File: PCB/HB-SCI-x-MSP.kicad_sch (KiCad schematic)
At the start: 31 parts, among them J1 Prog, J2 FTDI, Q1 BC858, SW1 Config, SW2 4x SW, U1 ATmega328P-AU, U2 MSP430F2001IPW, U3 CC1101, Y1 32kHz

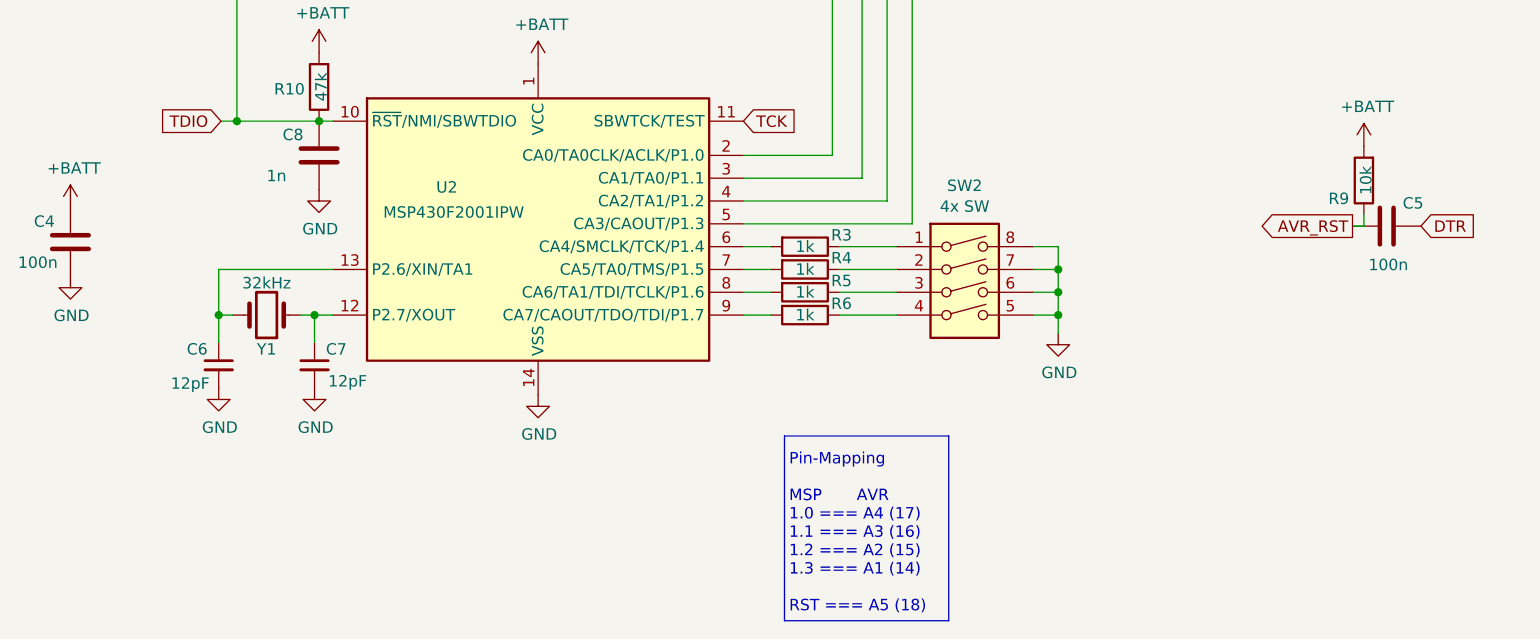
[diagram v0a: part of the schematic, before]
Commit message: update kicad
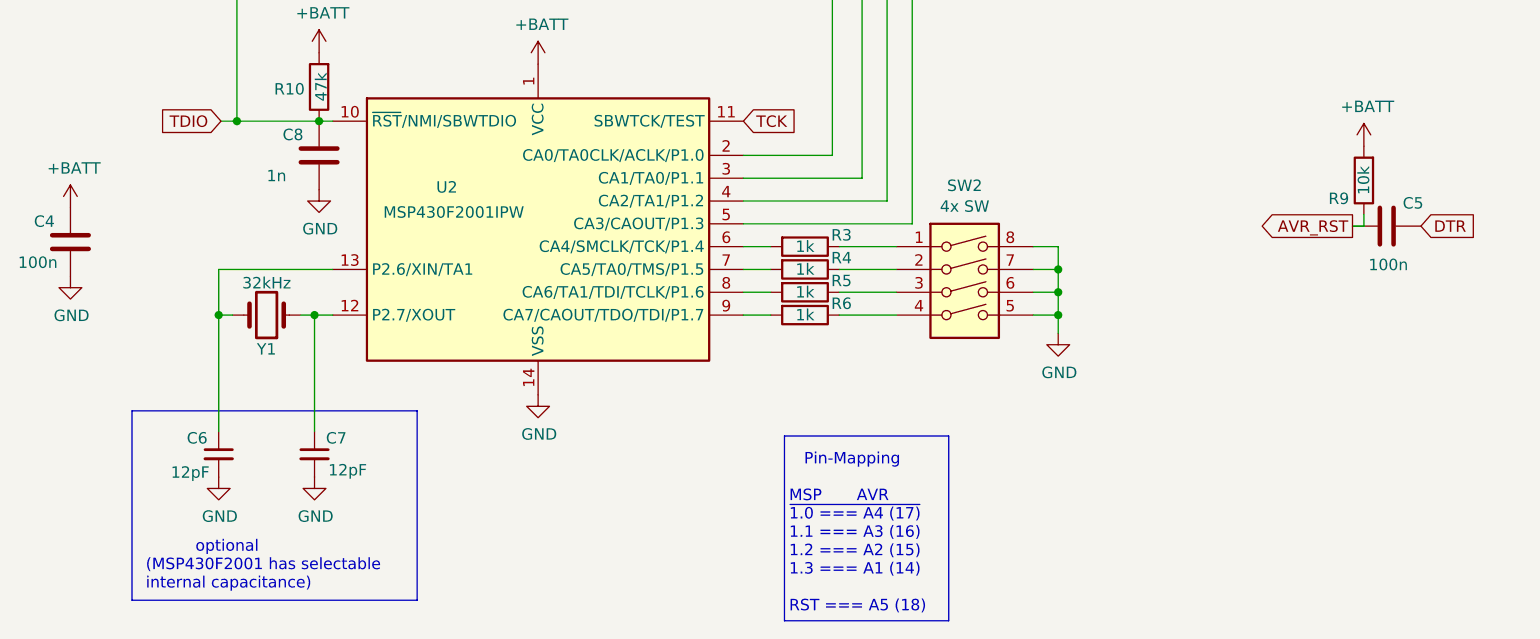
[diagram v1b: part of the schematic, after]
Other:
- note added: "Pin-Mapping MSP AVR ~{1.0 === A4 (17)} 1.1 === A3 (16) 1.2 === A2 (15) 1.3 === A1 (14) RST === A5 (18)"
- note added: "optional (MSP430F2001 has selectable internal capacitance)"
- note removed: "Pin-Mapping MSP AVR 1.0 === A4 (17) 1.1 === A3 (16) 1.2 === A2 (15) 1.3 === A1 (14) RST === A5 (18)"
- moved on the sheet: C6, C7
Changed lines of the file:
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@@
 (kicad_sch (version 20210621) (generator eeschema)
   (paper "A4")
-  (junction (at 43.688 137.668) (diameter 0) (color 0 0 0 0))
-  (junction (at 184.404 110.49) (diameter 0) (color 0 0 0 0))
-  (junction (at 177.546 48.006) (diameter 0) (color 0 0 0 0))
-  (junction (at 213.614 60.706) (diameter 0) (color 0 0 0 0))
-  (junction (at 52.324 159.258) (diameter 0) (color 0 0 0 0))
-  (junction (at 76.962 37.846) (diameter 0) (color 0 0 0 0))
-  (junction (at 79.502 37.846) (diameter 0) (color 0 0 0 0))
-  (junction (at 135.128 154.178) (diameter 0) (color 0 0 0 0))
   (junction (at 135.128 156.718) (diameter 0) (color 0 0 0 0))
   (junction (at 124.714 69.088) (diameter 0) (color 0 0 0 0))
   (junction (at 135.128 159.258) (diameter 0) (color 0 0 0 0))
-  (junction (at 52.832 137.668) (diameter 0) (color 0 0 0 0))
-  (junction (at 41.656 159.258) (diameter 0) (color 0 0 0 0))
+  (junction (at 184.404 110.49) (diameter 0) (color 0 0 0 0))
+  (junction (at 43.688 137.668) (diameter 0) (color 0 0 0 0))
+  (junction (at 52.324 159.258) (diameter 0) (color 0 0 0 0))
+  (junction (at 177.546 48.006) (diameter 0) (color 0 0 0 0))
+  (junction (at 79.502 37.846) (diameter 0) (color 0 0 0 0))
   (junction (at 177.546 61.976) (diameter 0) (color 0 0 0 0))
   (junction (at 177.546 41.148) (diameter 0) (color 0 0 0 0))
+  (junction (at 41.656 159.258) (diameter 0) (color 0 0 0 0))
+  (junction (at 76.962 37.846) (diameter 0) (color 0 0 0 0))
+  (junction (at 52.832 137.668) (diameter 0) (color 0 0 0 0))
+  (junction (at 213.614 60.706) (diameter 0) (color 0 0 0 0))
+  (junction (at 135.128 154.178) (diameter 0) (color 0 0 0 0))
   (no_connect (at 92.202 107.188))
   (no_connect (at 206.502 55.626))
@@
     (stroke (width 0) (type default) (color 0 0 0 0))
   )
-  (wire (pts (xy 41.656 159.258) (xy 41.656 162.306))
+  (wire (pts (xy 41.656 159.258) (xy 41.656 172.212))
     (stroke (width 0) (type default) (color 0 0 0 0))
   )
@@
     (stroke (width 0) (type default) (color 0 0 0 0))
   )
+  (polyline (pts (xy 32.004 169.926) (xy 32.004 191.008))
+    (stroke (width 0) (type default) (color 0 0 0 0))
+  )
+  (polyline (pts (xy 32.004 169.926) (xy 63.754 169.926))
+    (stroke (width 0) (type default) (color 0 0 0 0))
+  )
+  (polyline (pts (xy 63.754 191.008) (xy 32.004 191.008))
+    (stroke (width 0) (type default) (color 0 0 0 0))
+  )
+  (polyline (pts (xy 63.754 169.926) (xy 63.754 191.008))
+    (stroke (width 0) (type default) (color 0 0 0 0))
+  )
   (wire (pts (xy 132.334 151.638) (xy 135.128 151.638))
     (stroke (width 0) (type default) (color 0 0 0 0))
@@
     (stroke (width 0) (type default) (color 0 0 0 0))
   )
-  (wire (pts (xy 52.324 162.306) (xy 52.324 159.258))
+  (wire (pts (xy 52.324 172.212) (xy 52.324 159.258))
     (stroke (width 0) (type default) (color 0 0 0 0))
   )
@@
     (stroke (width 0) (type default) (color 0 0 0 0))
   )
-  (text "Pin-Mapping\n\nMSP       AVR\n1.0 === A4 (17)\n1.1 === A3 (16)\n1.2 === A2 (15)\n1.3 === A1 (14)\n\nRST === A5 (18)"
+  (text "   Pin-Mapping\n\nMSP       AVR\n~{1.0 === A4 (17)}\n1.1 === A3 (16)\n1.2 === A2 (15)\n1.3 === A1 (14)\n\nRST === A5 (18)"
     (at 105.156 192.532 0)
+    (effects (font (size 1.27 1.27)) (justify left bottom))
+  )
+  (text "          optional\n(MSP430F2001 has selectable \ninternal capacitance)"
+    (at 33.528 189.992 0)
     (effects (font (size 1.27 1.27)) (justify left bottom))
   )
@@
     (in_bom yes) (on_board yes)
     (property "Reference" "R9" (id 0) (at 166.37 146.304 0))
-    (property "Value" "10k" (id 1) (at 169.418 144.272 90))
+    (property "Value" "10k" (id 1) (at 169.164 144.272 90))
     (property "Footprint" "Resistor_SMD:R_0805_2012Metric_Pad1.15x1.40mm_HandSolder" (id 2) (at 170.942 144.272 90)
       (effects (font (size 1.27 1.27)) hide)
@@
     (pin "1")
   )
-  (symbol (lib_id "Device:C_Small") (at 41.656 164.846 0) (unit 1)
-    (in_bom yes) (on_board yes)
-    (property "Reference" "C6" (id 0) (at 38.1 163.068 0)
-      (effects (font (size 1.27 1.27)) (justify left))
-    )
-    (property "Value" "12pF" (id 1) (at 36.322 166.878 0)
-      (effects (font (size 1.27 1.27)) (justify left))
-    )
-    (property "Footprint" "Capacitor_SMD:C_0805_2012Metric_Pad1.15x1.40mm_HandSolder" (id 2) (at 41.656 164.846 0)
-      (effects (font (size 1.27 1.27)) hide)
-    )
-    (property "Datasheet" "~" (id 3) (at 41.656 164.846 0)
-      (effects (font (size 1.27 1.27)) hide)
-    )
-    (pin "1")
-    (pin "2")
-  )
-  (symbol (lib_id "Device:C_Small") (at 52.324 164.846 0) (unit 1)
-    (in_bom yes) (on_board yes)
-    (property "Reference" "C7" (id 0) (at 53.594 163.068 0)
-      (effects (font (size 1.27 1.27)) (justify left))
-    )
-    (property "Value" "12pF" (id 1) (at 53.848 166.624 0)
-      (effects (font (size 1.27 1.27)) (justify left))
-    )
-    (property "Footprint" "Capacitor_SMD:C_0805_2012Metric_Pad1.15x1.40mm_HandSolder" (id 2) (at 52.324 164.846 0)
-      (effects (font (size 1.27 1.27)) hide)
-    )
-    (property "Datasheet" "~" (id 3) (at 52.324 164.846 0)
-      (effects (font (size 1.27 1.27)) hide)
-    )
-    (pin "1")
-    (pin "2")
-  )
-  (symbol (lib_id "power:GND") (at 41.656 167.386 0) (unit 1)
-    (in_bom yes) (on_board yes)
-    (property "Reference" "#PWR03" (id 0) (at 41.656 173.736 0)
-      (effects (font (size 1.27 1.27)) hide)
-    )
-    (property "Value" "GND" (id 1) (at 41.783 171.7802 0))
-    (property "Footprint" "" (id 2) (at 41.656 167.386 0)
-      (effects (font (size 1.27 1.27)) hide)
-    )
-    (property "Datasheet" "" (id 3) (at 41.656 167.386 0)
-      (effects (font (size 1.27 1.27)) hide)
-    )
-    (pin "1")
-  )
-  (symbol (lib_id "power:GND") (at 52.324 167.386 0) (unit 1)
-    (in_bom yes) (on_board yes)
-    (property "Reference" "#PWR04" (id 0) (at 52.324 173.736 0)
-      (effects (font (size 1.27 1.27)) hide)
-    )
-    (property "Value" "GND" (id 1) (at 52.451 171.7802 0))
-    (property "Footprint" "" (id 2) (at 52.324 167.386 0)
-      (effects (font (size 1.27 1.27)) hide)
-    )
-    (property "Datasheet" "" (id 3) (at 52.324 167.386 0)
-      (effects (font (size 1.27 1.27)) hide)
-    )
+  (symbol (lib_id "Device:C_Small") (at 41.656 174.752 0) (unit 1)
+    (in_bom yes) (on_board yes)
+    (property "Reference" "C6" (id 0) (at 38.1 172.974 0)
+      (effects (font (size 1.27 1.27)) (justify left))
+    )
+    (property "Value" "12pF" (id 1) (at 36.322 176.784 0)
+      (effects (font (size 1.27 1.27)) (justify left))
+    )
+    (property "Footprint" "Capacitor_SMD:C_0805_2012Metric_Pad1.15x1.40mm_HandSolder" (id 2) (at 41.656 174.752 0)
+      (effects (font (size 1.27 1.27)) hide)
+    )
+    (property "Datasheet" "~" (id 3) (at 41.656 174.752 0)
+      (effects (font (size 1.27 1.27)) hide)
+    )
+    (pin "1")
+    (pin "2")
+  )
+  (symbol (lib_id "Device:C_Small") (at 52.324 174.752 0) (unit 1)
+    (in_bom yes) (on_board yes)
+    (property "Reference" "C7" (id 0) (at 53.594 172.974 0)
+      (effects (font (size 1.27 1.27)) (justify left))
+    )
+    (property "Value" "12pF" (id 1) (at 53.848 176.53 0)
+      (effects (font (size 1.27 1.27)) (justify left))
+    )
+    (property "Footprint" "Capacitor_SMD:C_0805_2012Metric_Pad1.15x1.40mm_HandSolder" (id 2) (at 52.324 174.752 0)
+      (effects (font (size 1.27 1.27)) hide)
+    )
+    (property "Datasheet" "~" (id 3) (at 52.324 174.752 0)
+      (effects (font (size 1.27 1.27)) hide)
+    )
+    (pin "1")
+    (pin "2")
+  )
+  (symbol (lib_id "power:GND") (at 41.656 177.292 0) (unit 1)
+    (in_bom yes) (on_board yes)
+    (property "Reference" "#PWR03" (id 0) (at 41.656 183.642 0)
+      (effects (font (size 1.27 1.27)) hide)
+    )
+    (property "Value" "GND" (id 1) (at 41.783 181.6862 0))
+    (property "Footprint" "" (id 2) (at 41.656 177.292 0)
+      (effects (font (size 1.27 1.27)) hide)
+    )
+    (property "Datasheet" "" (id 3) (at 41.656 177.292 0)
+      (effects (font (size 1.27 1.27)) hide)
+    )
+    (pin "1")
+  )
+  (symbol (lib_id "power:GND") (at 52.324 177.292 0) (unit 1)
+    (in_bom yes) (on_board yes)
+    (property "Reference" "#PWR04" (id 0) (at 52.324 183.642 0)
+      (effects (font (size 1.27 1.27)) hide)
+    )
+    (property "Value" "GND" (id 1) (at 52.451 181.6862 0))
+    (property "Footprint" "" (id 2) (at 52.324 177.292 0)
+      (effects (font (size 1.27 1.27)) hide)
+    )
+    (property "Datasheet" "" (id 3) (at 52.324 177.292 0)
+      (effects (font (size 1.27 1.27)) hide)
+    )
